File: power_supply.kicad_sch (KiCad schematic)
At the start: 11 parts, among them J6 USB4510-03-1-A, U2 LP5907MFX-3.3/NOPB, U3 LMC7660IMX/NOPB

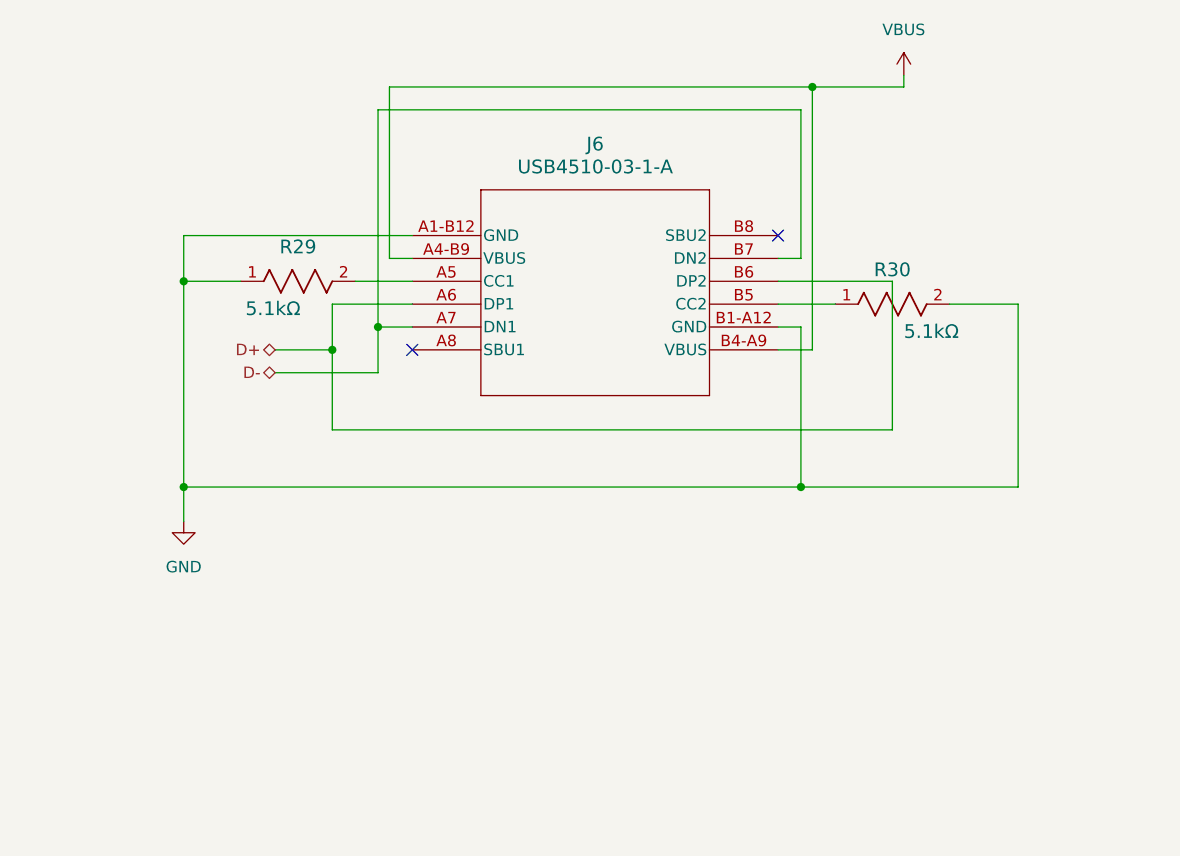
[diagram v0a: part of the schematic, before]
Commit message: pcb almost done, just need to do the final copper fill
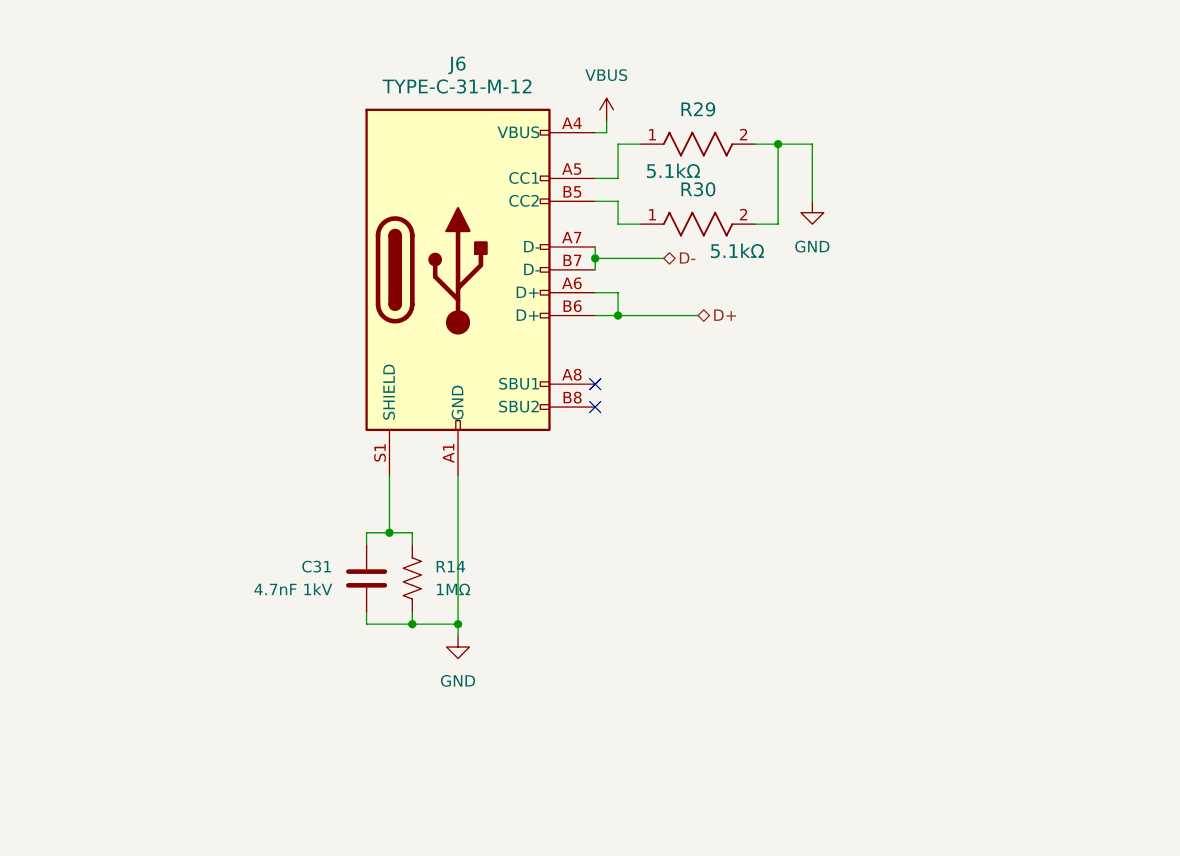
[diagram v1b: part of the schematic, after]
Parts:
- added C31: 4.7nF 1kV, Capacitor_SMD:C_1206_3216Metric, symbol Device:C
- added R14: 1MΩ, Resistor_SMD:R_2512_6332Metric, symbol Device:R_US
- J6: value USB4510-03-1-A -> TYPE-C-31-M-12; footprint CMPE2750:USB4510-03-1-A_GCT -> Connector_USB:USB_C_Receptacle_HRO_TYPE-C-31-M-12; symbol CMPE2750:USB4510-03-1-A -> Connector:USB_C_Receptacle_USB2.0_16P
- U2: footprint DBV0005A_N -> CMPE2750:DBV0005A_N
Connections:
- net GND: now also J6.A1 (GND), J6.A12 (GND), J6.B1 (GND), J6.B12 (GND), R29.2, C31.2, R14.2; no longer J6.A1-B12 (GND), J6.B1-A12 (GND), R29.1
- net VBUS: now also J6.A4 (VBUS), J6.A9 (VBUS), J6.B4 (VBUS), J6.B9 (VBUS); no longer J6.A4-B9 (VBUS), J6.B4-A9 (VBUS)
- net at J6.A5 (CC1): now also R29.1; no longer R29.2
- new net: C31.1, J6.S1 (SHIELD), R14.1
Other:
- moved on the sheet: R29, R30
